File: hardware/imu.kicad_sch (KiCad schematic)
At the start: 4 parts, among them U9 LSM6DSV16XTR

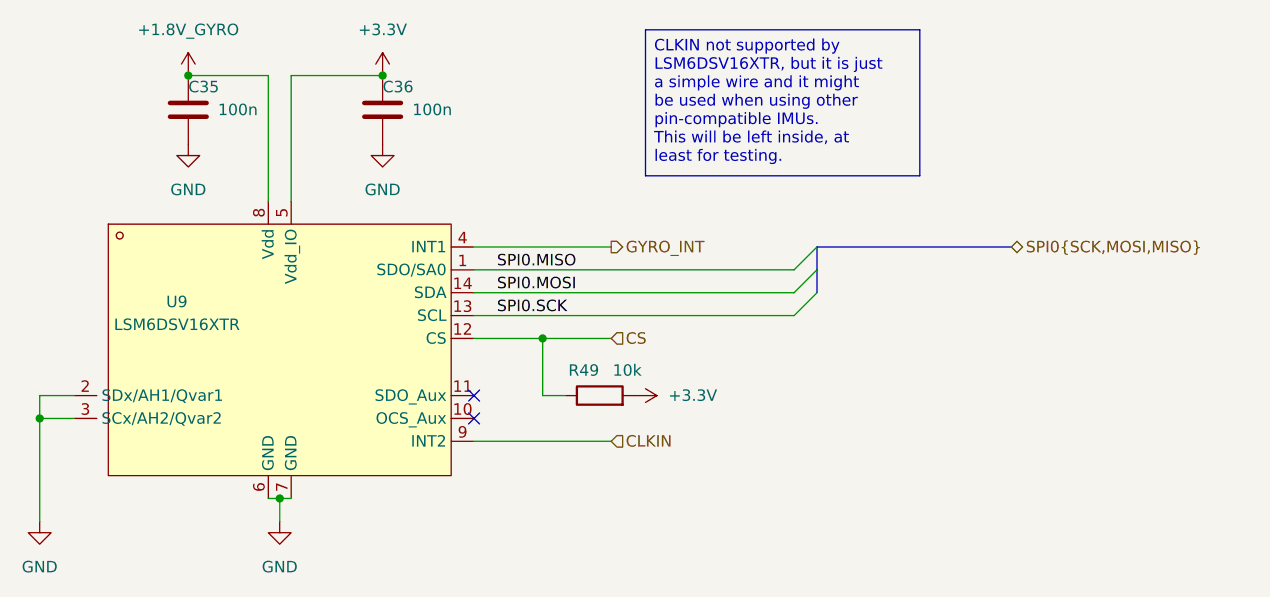
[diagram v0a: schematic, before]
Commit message: switch spi
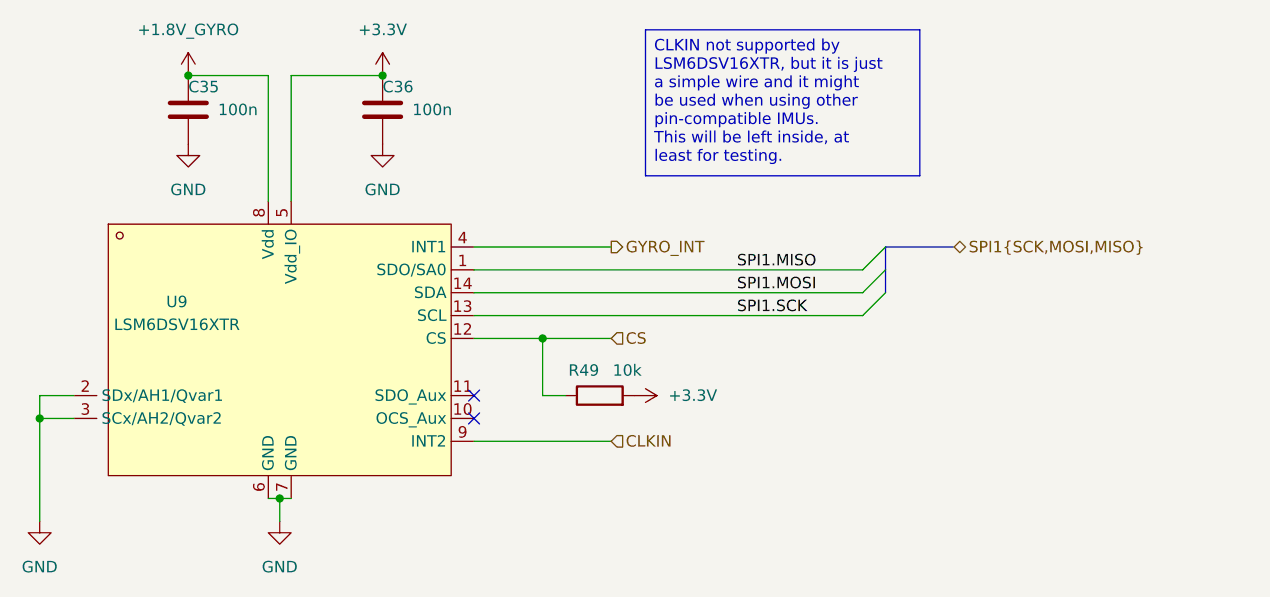
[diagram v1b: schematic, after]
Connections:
- net SPI0.MISO renamed SPI1.MISO
- net SPI0.MOSI renamed SPI1.MOSI
- net SPI0.SCK renamed SPI1.SCK
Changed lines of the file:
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@@
 	)
 	(bus_entry
-		(at 129.54 67.31)
+		(at 137.16 64.77)
 		(size 2.54 -2.54)
 		(stroke
@@
 	)
 	(bus_entry
-		(at 129.54 64.77)
+		(at 137.16 69.85)
 		(size 2.54 -2.54)
 		(stroke
@@
 	)
 	(bus_entry
-		(at 129.54 69.85)
+		(at 137.16 67.31)
 		(size 2.54 -2.54)
 		(stroke
@@
 		)
 	)
-	(wire
-		(pts
-			(xy 93.98 64.77) (xy 129.54 64.77)
+	(bus
+		(pts
+			(xy 139.7 64.77) (xy 139.7 67.31)
 		)
 		(stroke
@@
 		)
 	)
-	(wire
-		(pts
-			(xy 93.98 69.85) (xy 129.54 69.85)
+	(bus
+		(pts
+			(xy 139.7 62.23) (xy 139.7 64.77)
+		)
+		(stroke
+			(width 0)
+			(type default)
+		)
+	)
+	(bus
+		(pts
+			(xy 147.32 62.23) (xy 139.7 62.23)
 		)
 		(stroke
@@
 	(wire
 		(pts
+			(xy 93.98 64.77) (xy 137.16 64.77)
+		)
+		(stroke
+			(width 0)
+			(type default)
+		)
+	)
+	(wire
+		(pts
+			(xy 93.98 67.31) (xy 137.16 67.31)
+		)
+		(stroke
+			(width 0)
+			(type default)
+		)
+	)
+	(wire
+		(pts
 			(xy 93.98 62.23) (xy 109.22 62.23)
 		)
@@
 		)
 	)
-	(bus
-		(pts
-			(xy 132.08 64.77) (xy 132.08 62.23)
-		)
-		(stroke
-			(width 0)
-			(type default)
-		)
-	)
 	(wire
 		(pts
@@
 		)
 	)
-	(bus
-		(pts
-			(xy 132.08 62.23) (xy 153.67 62.23)
-		)
-		(stroke
-			(width 0)
-			(type default)
-		)
-	)
 	(wire
 		(pts
@@
 		)
 	)
-	(bus
-		(pts
-			(xy 132.08 67.31) (xy 132.08 64.77)
-		)
-		(stroke
-			(width 0)
-			(type default)
-		)
-	)
 	(wire
 		(pts
@@
 	(wire
 		(pts
-			(xy 93.98 67.31) (xy 129.54 67.31)
-		)
-		(stroke
-			(width 0)
-			(type default)
-		)
-	)
-	(wire
-		(pts
 			(xy 45.72 78.74) (xy 49.53 78.74)
 		)
@@
 	(wire
 		(pts
+			(xy 93.98 69.85) (xy 137.16 69.85)
+		)
+		(stroke
+			(width 0)
+			(type default)
+		)
+	)
+	(wire
+		(pts
 			(xy 71.12 43.18) (xy 71.12 57.15)
 		)
@@
 		)
 	)
-	(label "SPI0.MOSI"
-		(at 96.52 67.31 0)
+	(label "SPI1.MISO"
+		(at 123.19 64.77 0)
 		(effects
 			(font
@@
 		)
 	)
-	(label "SPI0.MISO"
-		(at 96.52 64.77 0)
+	(label "SPI1.MOSI"
+		(at 123.19 67.31 0)
 		(effects
 			(font
@@
 		)
 	)
-	(label "SPI0.SCK"
-		(at 96.52 69.85 0)
+	(label "SPI1.SCK"
+		(at 123.19 69.85 0)
 		(effects
 			(font
@@
 			)
 			(justify left bottom)
+		)
+	)
+	(hierarchical_label "SPI1{SCK,MOSI,MISO}"
+		(shape bidirectional)
+		(at 147.32 62.23 0)
+		(effects
+			(font
+				(size 1.27 1.27)
+			)
+			(justify left)
 		)
 	)
@@
 		(effects
 			(font
-				(size 1.27 1.27)
-			)
-			(justify left)
-		)
-	)
-	(hierarchical_label "SPI0{SCK,MOSI,MISO}"
-		(shape bidirectional)
-		(at 153.67 62.23 0)
-		(effects
-			(font
